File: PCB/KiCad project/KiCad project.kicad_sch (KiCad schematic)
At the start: 7 parts, among them SW2 SW_Push, SW3 SW_Push, SW4 SW_Push, U1 XIAO-RP2040-DIP, U2 OLED_0.91_128x32

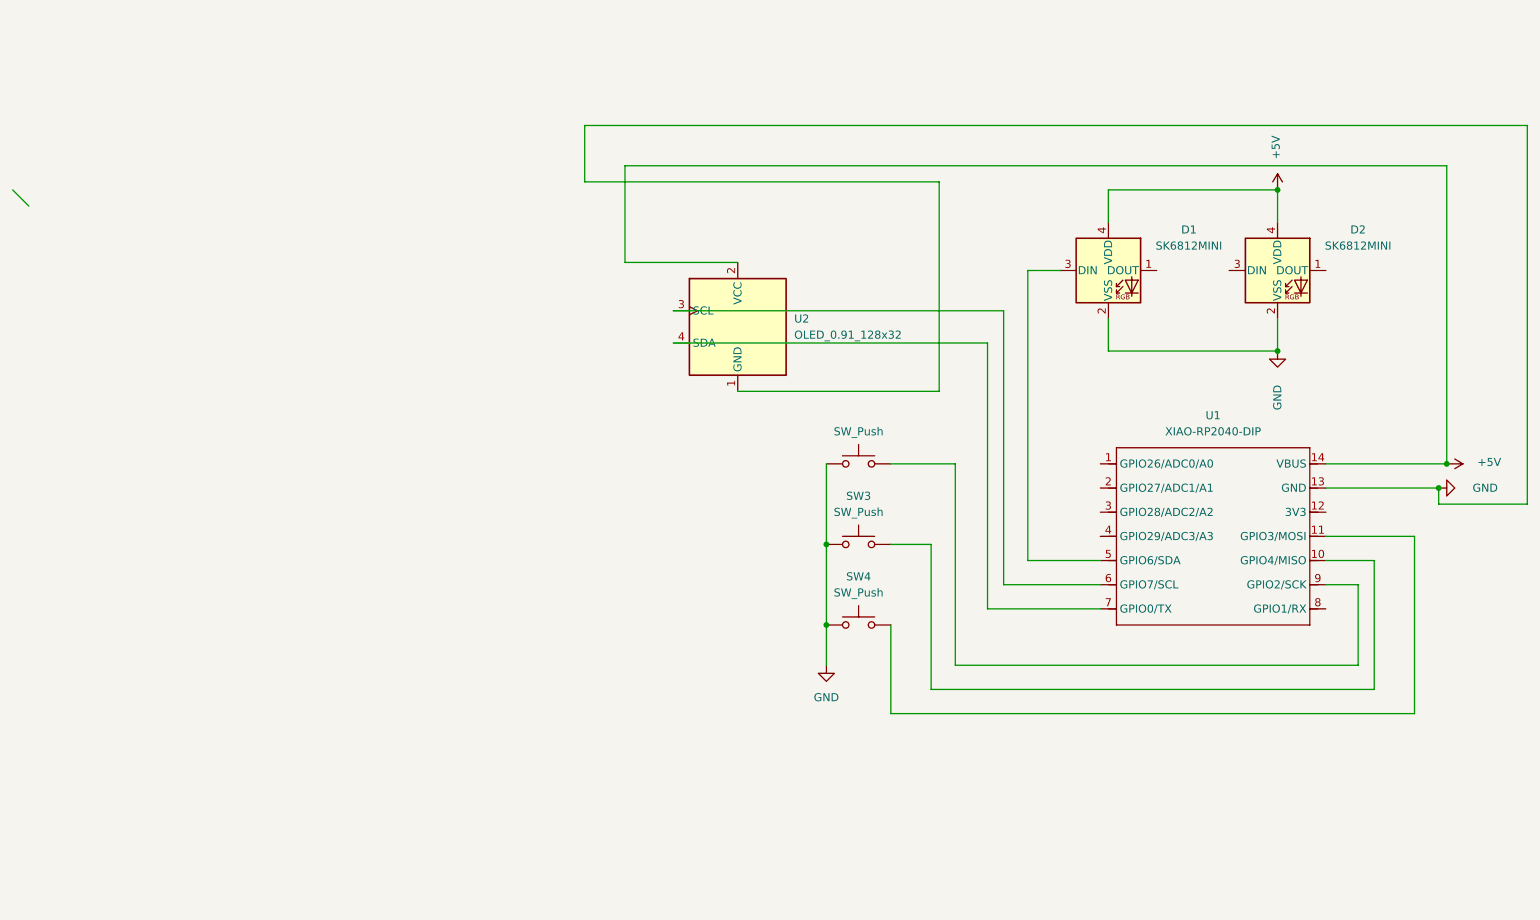
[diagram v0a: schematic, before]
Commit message: Add files via upload
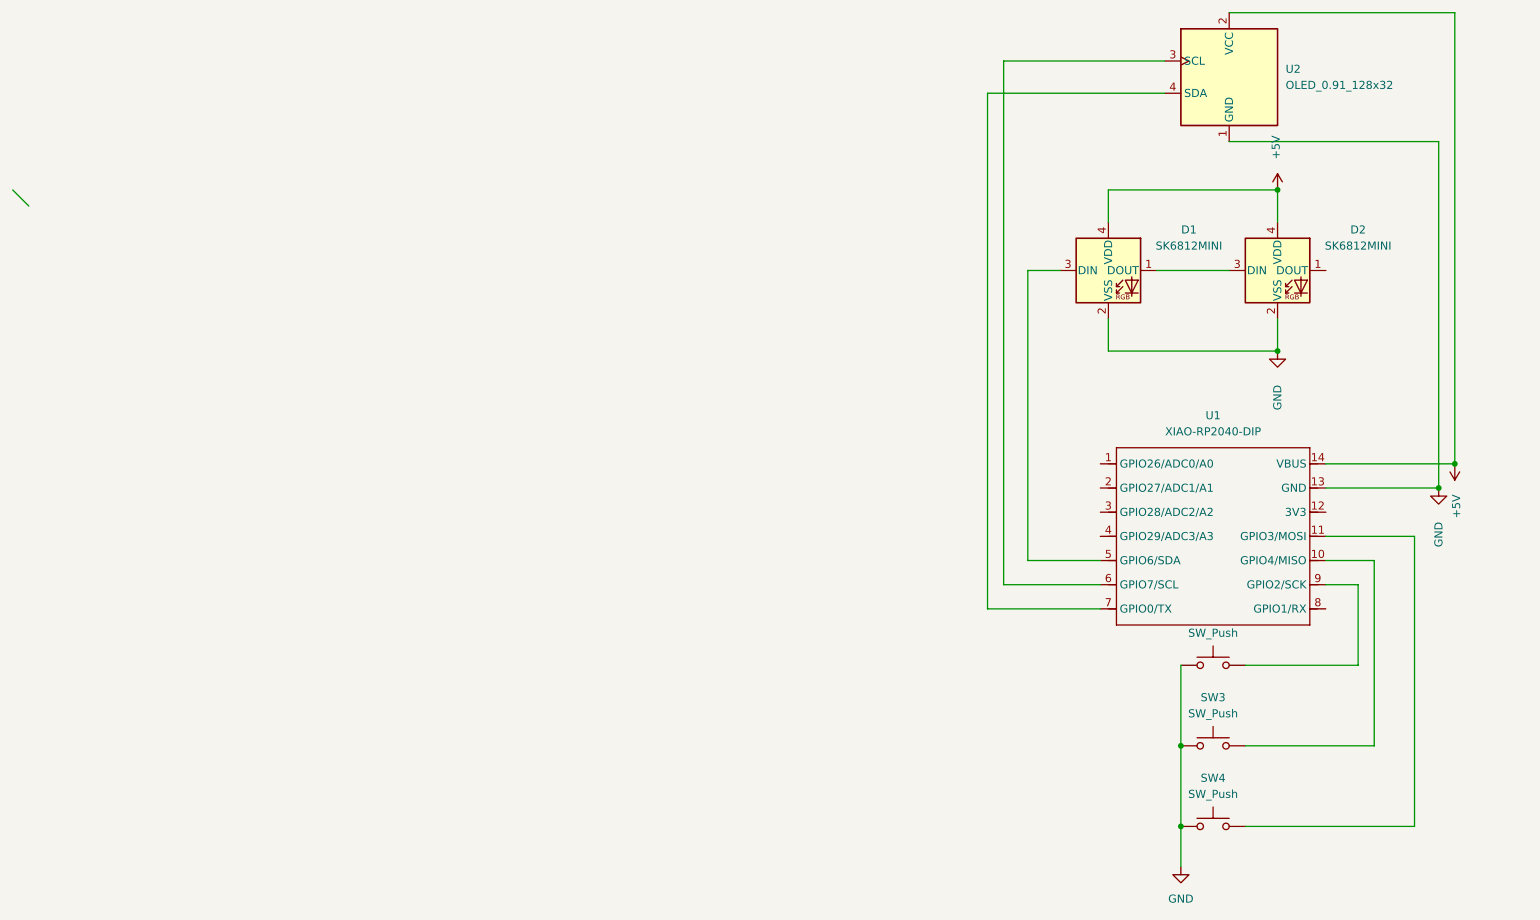
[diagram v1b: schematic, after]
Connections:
- net at D2.3 (DIN): now also D1.1 (DOUT)
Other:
- moved on the sheet: SW3, SW4, U2
